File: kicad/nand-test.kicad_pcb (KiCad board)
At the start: 2 copper layers, 48.3 x 33 mm, 9 parts, among them J1 PWR, Q1 2N3904, Q2 2N3904, SW1 SW_SPST, SW2 SW_SPST

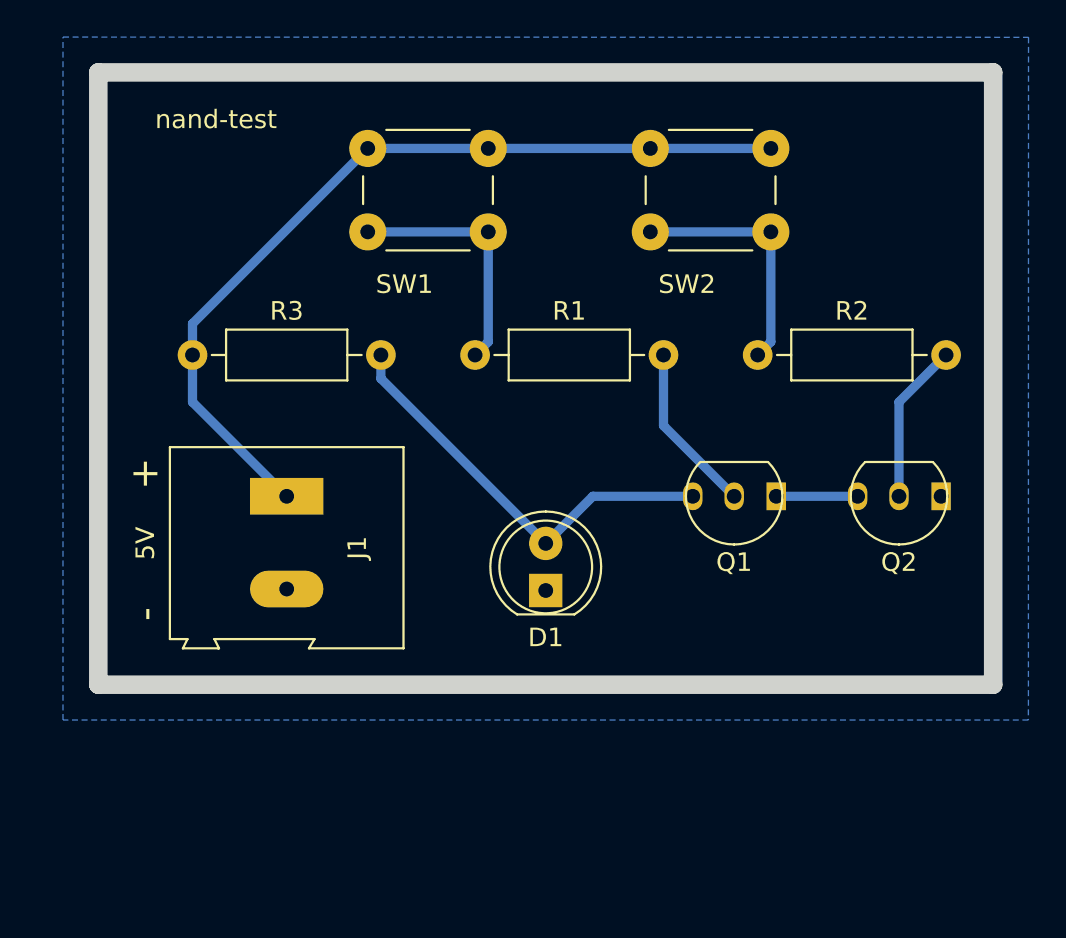
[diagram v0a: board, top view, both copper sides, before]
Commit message: updates gerbers, gcode, and notes
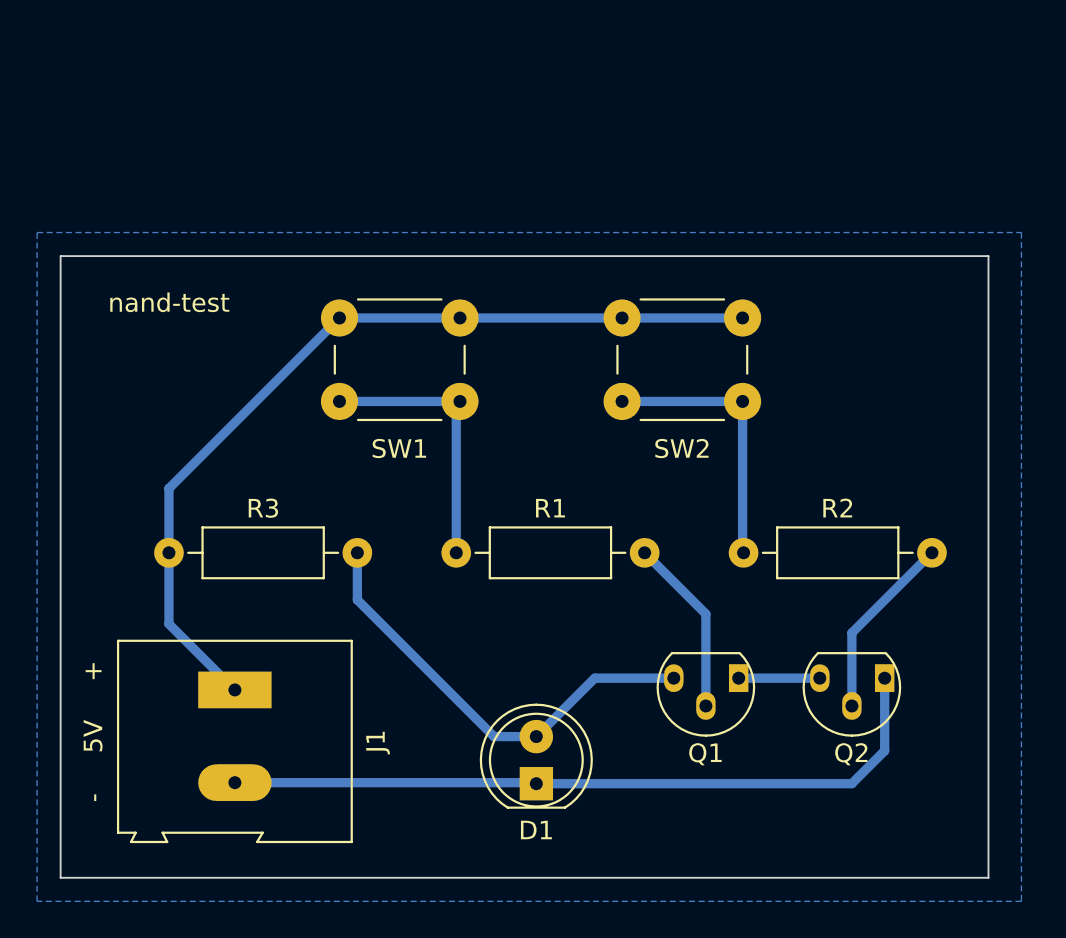
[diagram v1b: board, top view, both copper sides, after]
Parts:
- moved J1 10.8 mm to (88.6, 89.2)
- moved R3 10.7 mm to (85.1, 81.8)
- moved R1 10.7 mm to (100.6, 81.8)
- moved R2 10.7 mm to (116.1, 81.8)
- moved Q2 10.6 mm to (123.2, 89.0)
- moved D1 10.4 mm to (104.9, 94.2)
- moved Q1 10.4 mm to (115.3, 89.0)
- moved SW1 9.27 mm to (94.3, 69.1)
- moved SW2 9.27 mm to (109.5, 69.1)
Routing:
- net GND: track 0.11 -> 39.7 mm
- net Net-(Q2-Pad2): track 8.67 -> 10.0 mm
- net Net-(R1-Pad1): track 13.4 -> 14.7 mm
- net Net-(R2-Pad1): track 13.4 -> 14.7 mm
- net Net-(D1-Pad2): track 22.8 -> 24.0 mm
- net +5V: track 46.5 -> 47.1 mm
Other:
- board size 48.3 x 33 mm -> 50 x 33.5 mm
